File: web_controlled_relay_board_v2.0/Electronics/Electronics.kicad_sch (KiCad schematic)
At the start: 69 parts, among them J1 Screw_Terminal_01x10, J2 Screw_Terminal_01x10, J3 Screw_Terminal_01x02, J4 Screw_Terminal_01x02, K1 G3MB-202P, K10 G3MB-202P, K11 G3MB-202P, K12 G3MB-202P, K13 G3MB-202P, K14 G3MB-202P, K15 G3MB-202P, K16 G3MB-202P, K17 G3MB-202P, K18 G3MB-202P, K19 G3MB-202P, K2 G3MB-202P, K20 G3MB-202P, K3 G3MB-202P, K4 G3MB-202P, K5 G3MB-202P, K6 G3MB-202P, K7 G3MB-202P, K8 G3MB-202P, K9 G3MB-202P, SW1 SW_MEC_5E, U1 PC817, U10 PC817, U11 PC817, U12 PC817, U13 PC817, U14 PC817, U15 PC817, U16 PC817, U17 PC817, U18 PC817, U19 PC817, U2 PC817, U20 PC817, U3 PC817, U4 PC817, U5 PC817, U6 PC817, U7 PC817, U8 PC817, U9 PC817

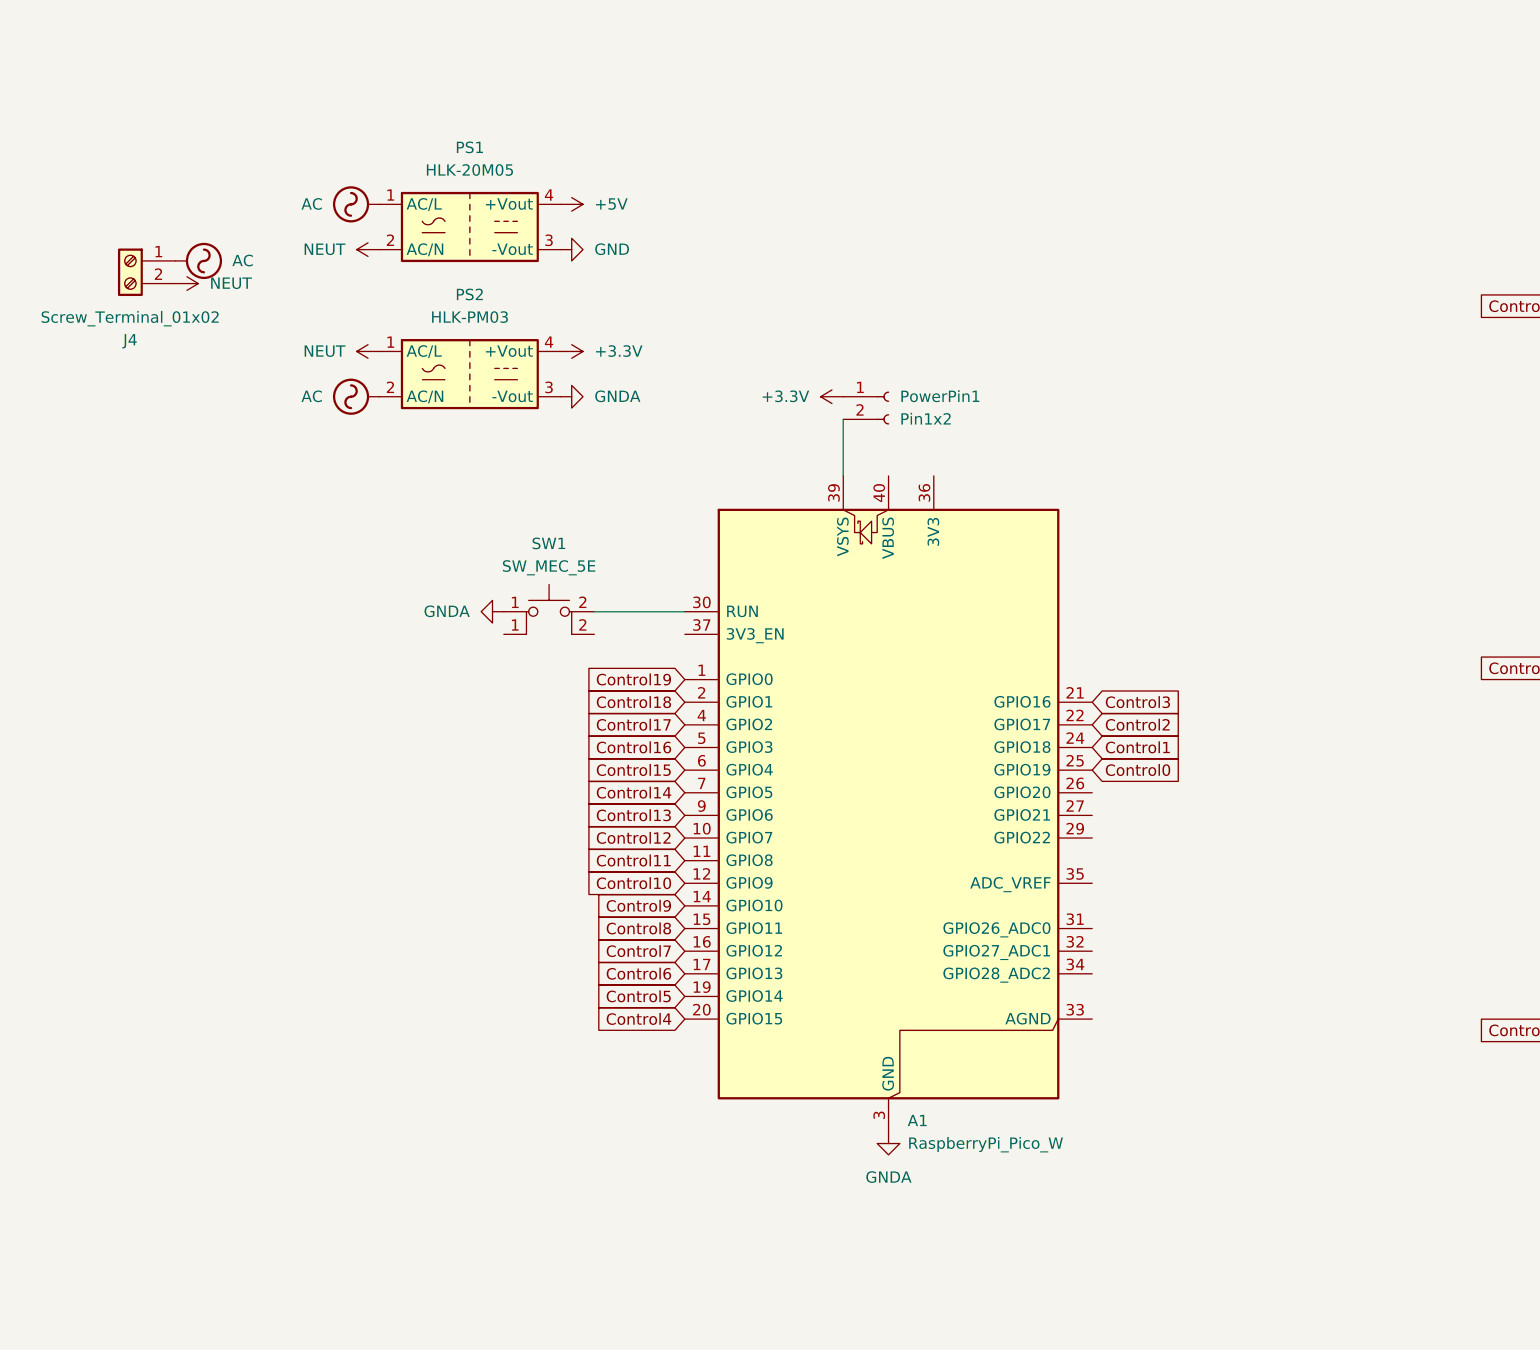
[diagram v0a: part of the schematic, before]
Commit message: finished final touches of PCB schematic and layout
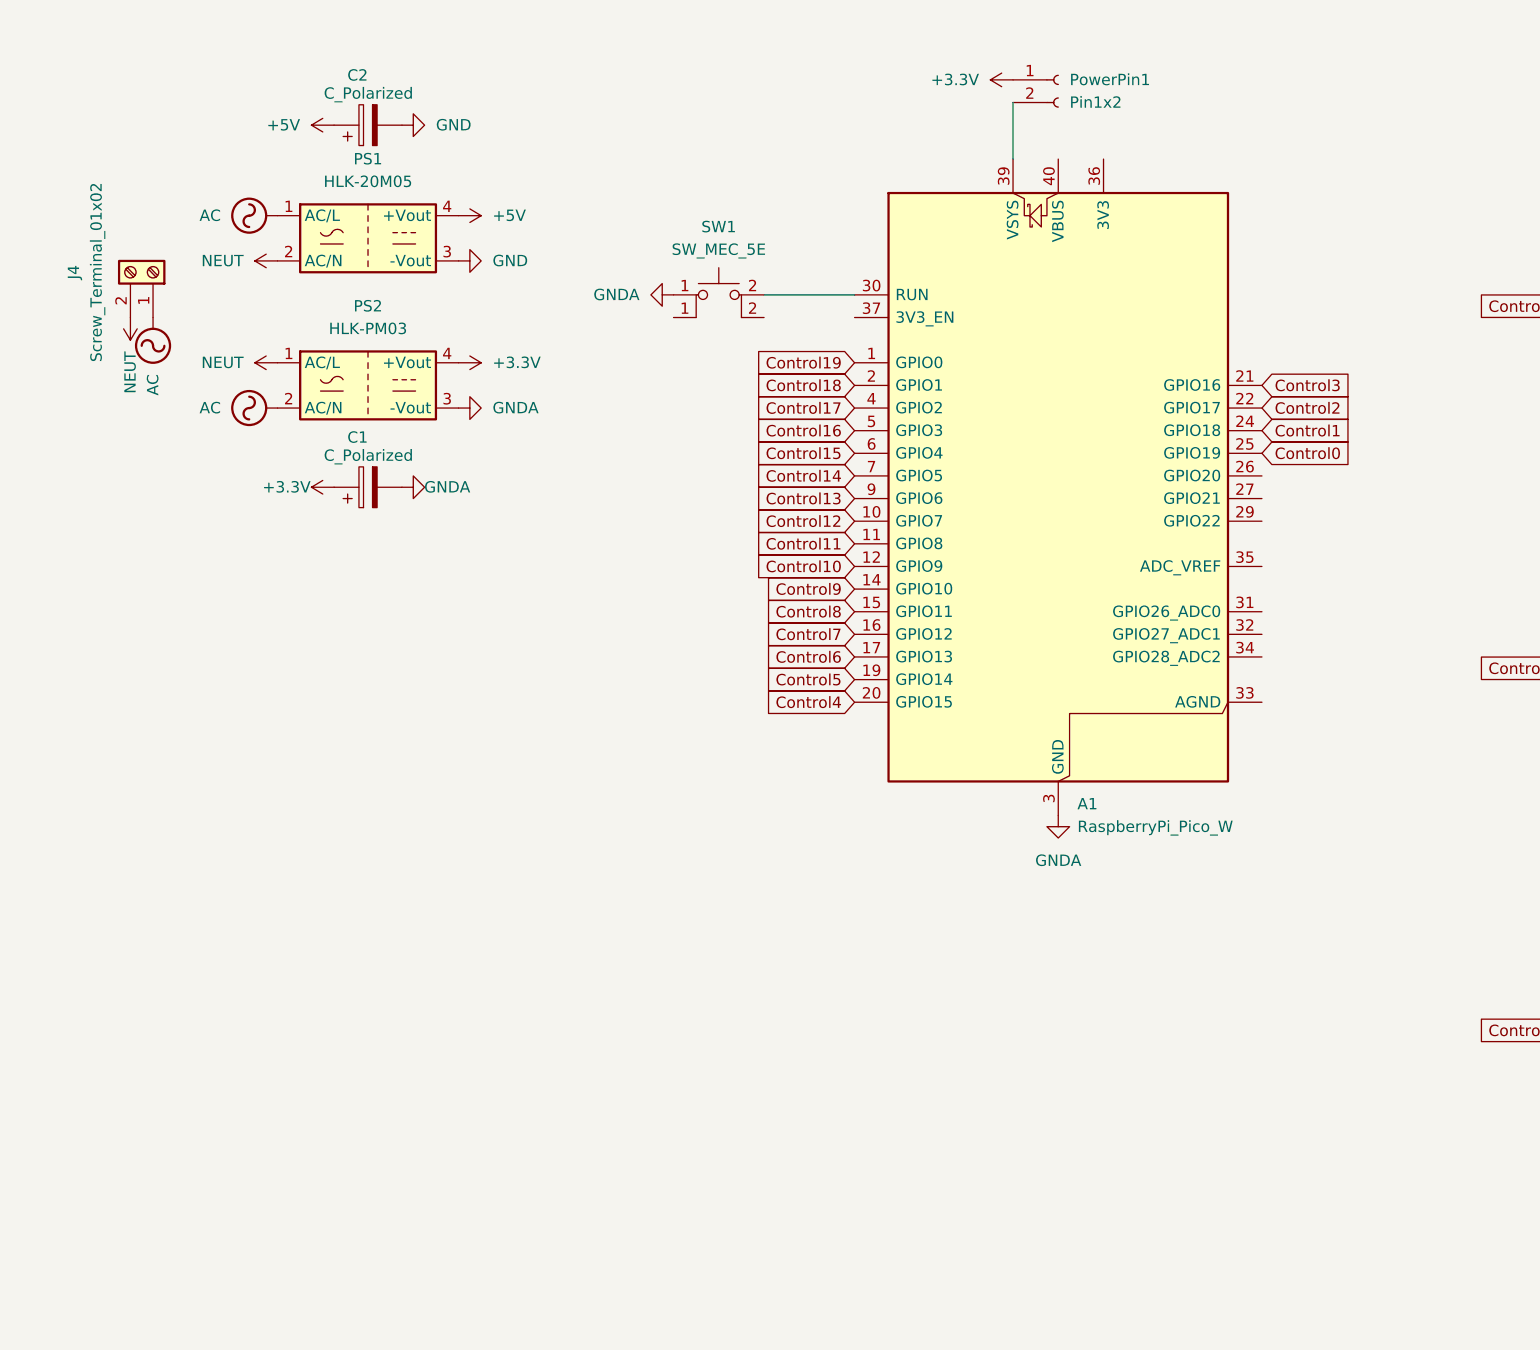
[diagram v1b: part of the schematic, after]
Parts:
- added C1: C_Polarized, Capacitor_THT:CP_Radial_D6.3mm_P2.50mm, symbol Device:C_Polarized
- added C2: C_Polarized, Capacitor_THT:CP_Radial_D8.0mm_P3.50mm, symbol Device:C_Polarized
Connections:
- net +3.3V: now also C1.1
- net +5V: now also C2.1
- net GND: now also C2.2
- net GNDA: now also C1.2
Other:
- moved on the sheet: A1, J4, PS1, PS2, PowerPin1, SW1
